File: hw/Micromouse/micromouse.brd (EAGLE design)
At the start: 160 x 100 mm, 48 parts, among them IC1 DSPIC33FJ64MC804-PT, IC2 DRV8833PWR, SW1 B3F-1000, SW2 B3F-1000, SW3 B3F-1000, T1 NHDTC1X4ETR, T2 NHDTC1X4ETR, T3 NHDTC1X4ETR, T4 NHDTC1X4ETR

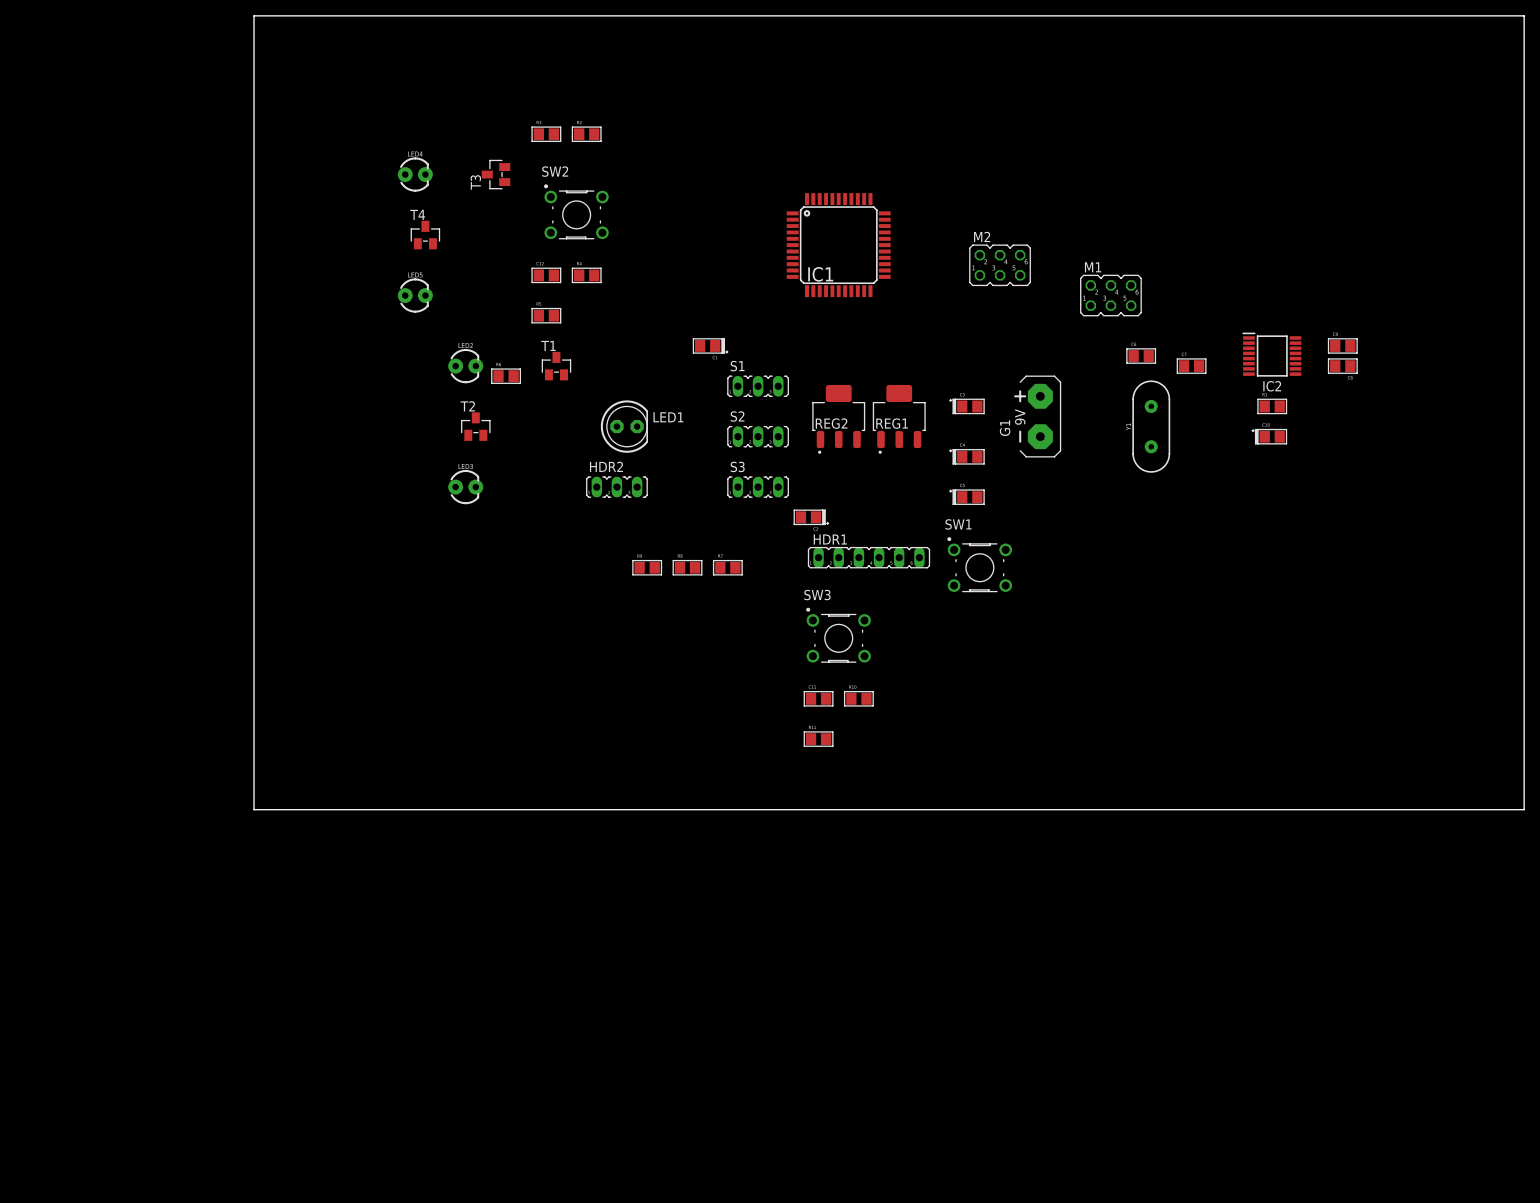
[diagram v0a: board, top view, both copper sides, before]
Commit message: Updated EAGLE project
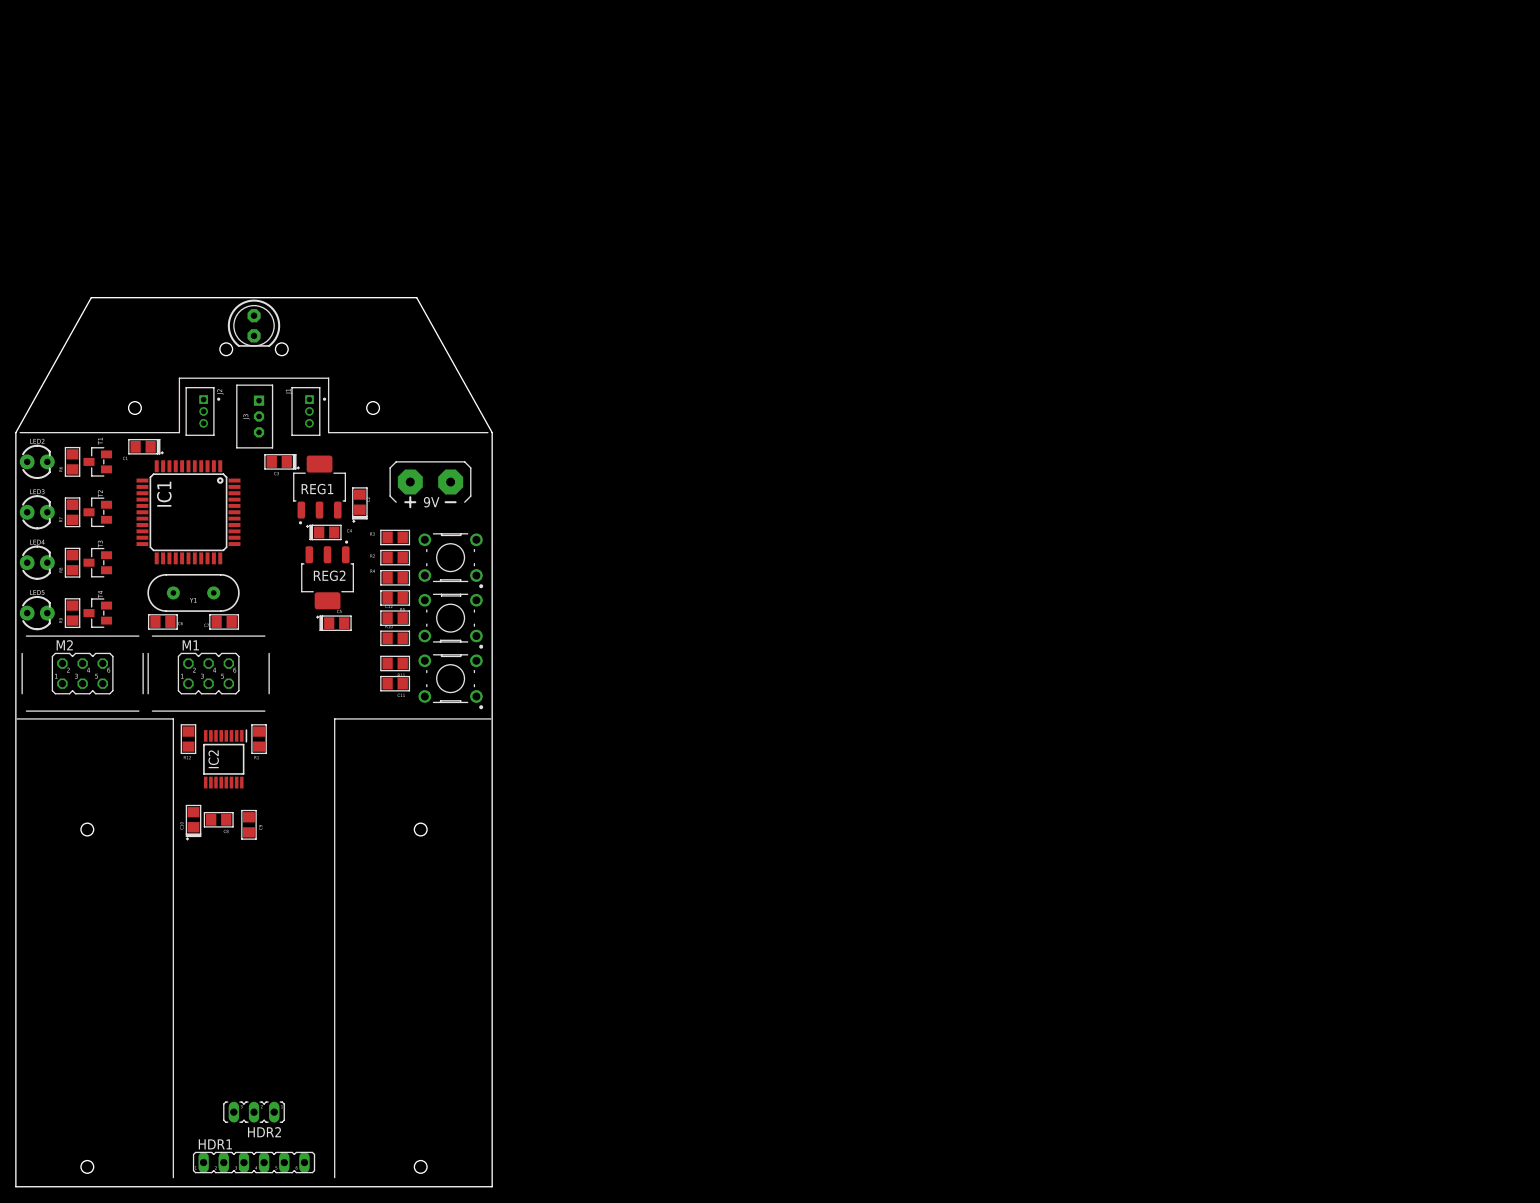
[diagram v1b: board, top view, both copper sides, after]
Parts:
- removed S1, S3: GP2Y0A51SK0F, micromouse:JP2Y
- removed S2: GP2Y0A41SK0F, micromouse:JP2Y
- added J1, J2: GP2Y0A51SK0F, micromouse:B3B-ZR(LF)(SN)
- added J3: GP2Y0A41SK0F, micromouse:B3B-PH-K-S
- added R12: 0.2, micromouse:0805
- moved C8 152.7 mm to (-4.45, -1.27)
- moved C9 150.4 mm to (-0.64, -1.91), turned to 270 degrees
- moved C10 144.2 mm to (-7.62, -1.27), turned to 90 degrees
- moved IC2 141.5 mm to (-3.81, 6.35), turned to 270 degrees
- moved R1 134.3 mm to (0.64, 8.89), turned to 270 degrees
- moved C6 127.7 mm to (-11.5, 23.6), turned to 180 degrees
- moved M2 126.5 mm to (-21.6, 17.1)
- moved C7 126.1 mm to (-3.76, 23.6)
- moved M1 123.2 mm to (-5.71, 17.1)
- moved Y1 122.5 mm to (-7.62, 27.3), turned to 180 degrees
- moved HDR1 108.7 mm to (-3.81, -44.5)
- moved HDR2 91.1 mm to (0.00, -38.1), turned to 180 degrees
- moved IC1 88.6 mm to (-8.26, 37.5), turned to 270 degrees
- moved C3 87.3 mm to (3.17, 43.8), turned to 180 degrees
- moved R7 82.8 mm to (-22.9, 37.5), turned to 90 degrees
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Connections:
- new net N$1: IC2.6, R12.1
- net +5V: now also J1.1, J2.1, J3.3; no longer S1.3, S2.1, S3.3
- net GND: now also J1.2, J2.2, J3.2, R12.2; no longer S1.2, S2.2, S3.2
- net N$5: no longer IC2.6
- net S1_OUT: now also J1.3; no longer S1.1
- net S2_OUT: now also J3.1; no longer S2.3
- net S3_OUT: now also J2.3; no longer S3.1
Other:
- board size 160 x 100 mm -> 60 x 112 mm
